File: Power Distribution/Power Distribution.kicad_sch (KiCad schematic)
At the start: 12 parts, among them P1 Charging/BoostConverterBoardT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, SW1 Switch, U1 Raspberry Pi Zero 2 W, U5 IMU BNO55

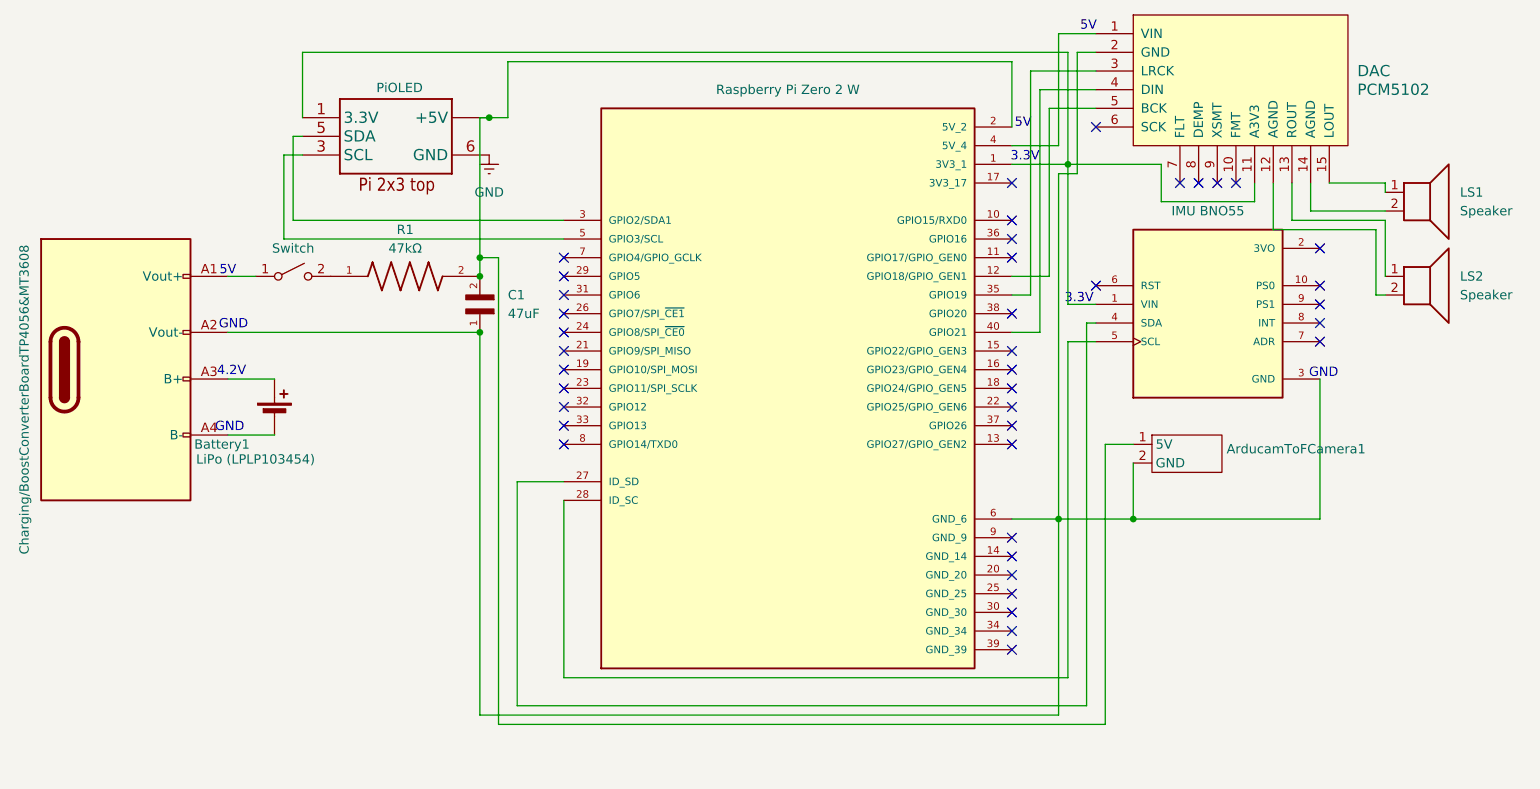
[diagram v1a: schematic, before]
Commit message: PCB update
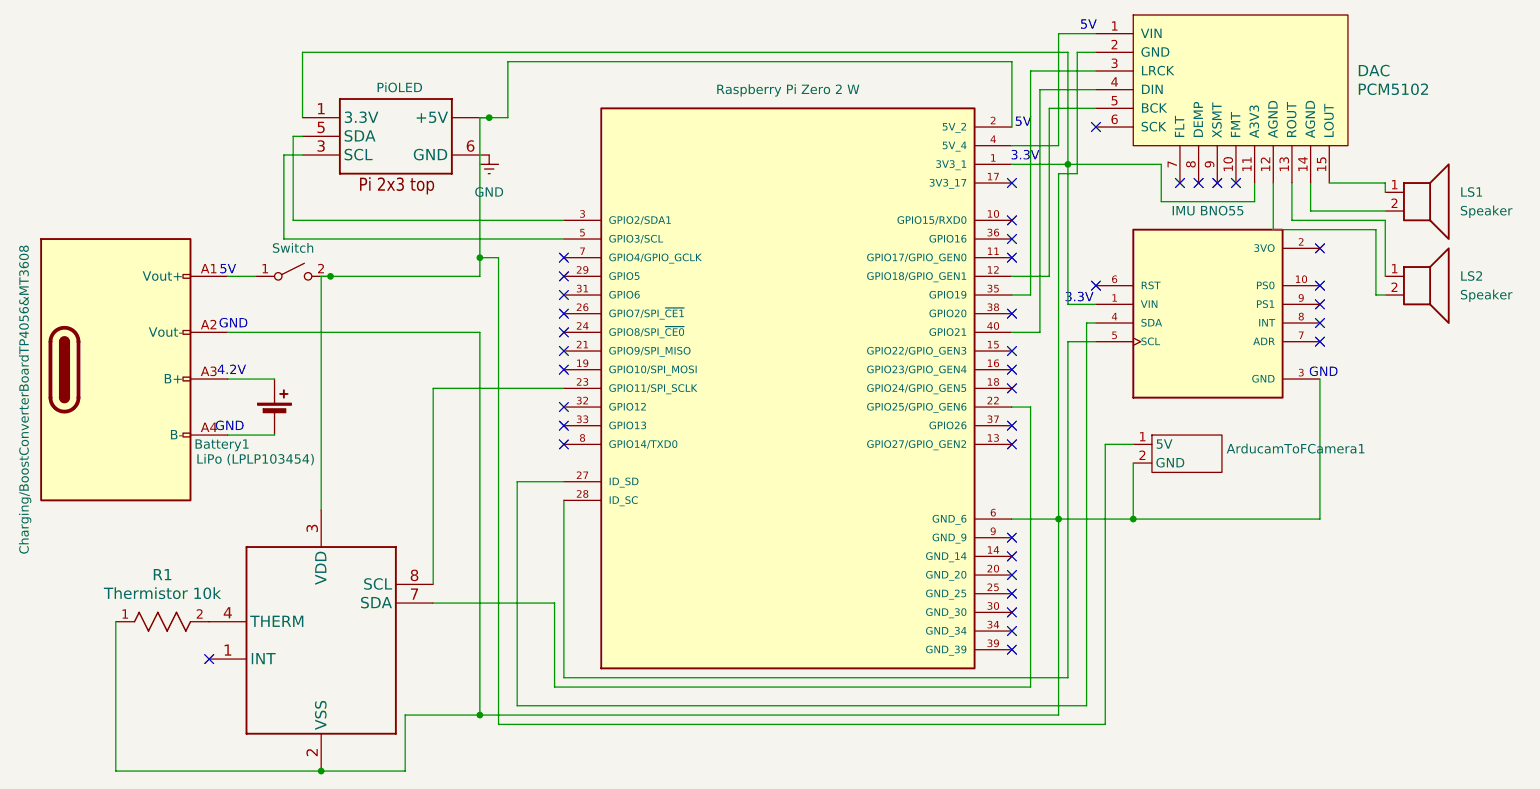
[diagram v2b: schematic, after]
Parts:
- removed C1: 47uF, 47uF:CAPC3225X280N, symbol GCJ32ER70J476KE01L:GCJ32ER70J476KE01L
- removed R1: 47kΩ, 47k:RES_ERA6ARW473V, symbol ERA6ARW473V:ERA6ARW473V
- added 1: ~, Adafruit LC709203F LiPoly LiIon Fuel Gauge and Battery Monitor:WDFN8_3X4_0.65, symbol LC709203F:LC709203F
- added R1: Thermistor 10k, RES_NCU15X_MUR, symbol Thermistor 10k:NCU15XH103F6SRC
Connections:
- net at ArducamToFCamera1.2 (GND), DAC.2 (GND), P1.A2 (Vout-)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: now also 1.2 (VSS), R1.1
- net at SW1.2 (B): now also ArducamToFCamera1.1 (5V), PiOLED.2 (+5V), PiOLED.4 (+5V), U1.2 (5V_2), 1.3 (VDD)
- net at U1.22 (GPIO25/GPIO_GEN6): now also 1.7 (SDA)
- net at U1.23 (GPIO11/SPI_SCLK): now also 1.8 (SCL)
- new net: 1.4 (THERM), R1.2
- no-connect marks 40 -> 39
